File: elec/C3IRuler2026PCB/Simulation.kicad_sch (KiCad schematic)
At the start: 4 parts

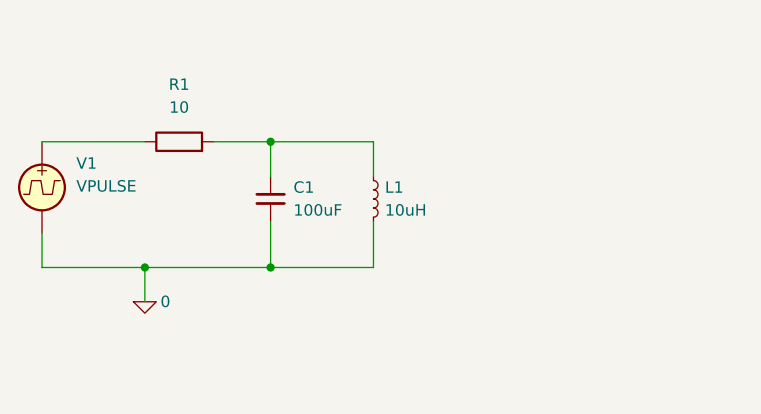
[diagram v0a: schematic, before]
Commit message: Experimenting with a square wave oscillator from an op-amp
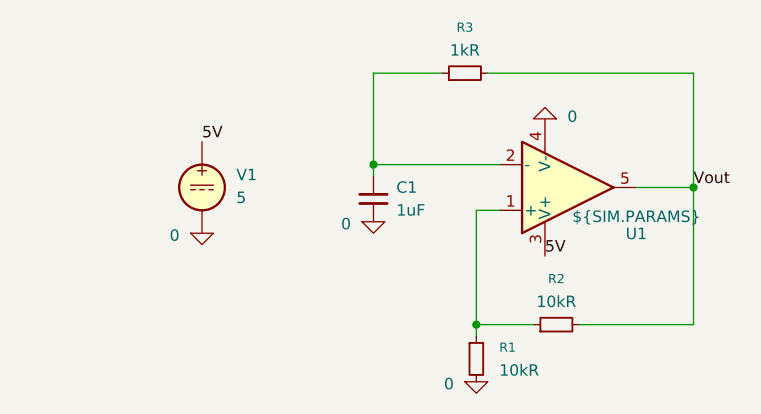
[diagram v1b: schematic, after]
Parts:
- removed L1: 10uH, symbol Device:L_Small
- removed R1: 10, symbol Device:R
- removed V1: VPULSE, symbol Simulation_SPICE:VPULSE
- added R1, R2: 10kR, symbol Device:R_Small
- added R3: 1kR, symbol Device:R_Small
- added U1: ${SIM.PARAMS}, symbol Simulation_SPICE:OPAMP
- added V1: 5, symbol Simulation_SPICE:VDC
- C1: value 100uF -> 1uF
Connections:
- net 0: now also R1.2, U1.4 (V-), V1.2
- net at C1.1: now also R3.1, U1.2 (-)
- new net: R1.1, R2.1, U1.1 (+)
- new net 5V: U1.3 (V+), V1.1
- new net Vout: R2.2, R3.2, U1.5
